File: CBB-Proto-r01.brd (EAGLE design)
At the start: 86.4 x 54.6 mm, 21 parts, among them IC1 IC16_SOIC, IC2 IC6_SOT23, IC4 IC6_SOT23, J1 HEADER_1X23, J10 HEADER_1X3, J11 HEADER_1X3, J12 HEADER_1X3, J13 HEADER_1X8, J14 HEADER_1X8, J15 HEADER_1X8, J16 HEADER_1X8, J2 HEADER_1X23, J3 HEADER_1X23, J4 HEADER_1X23, J5 HEADER_1X4, J6 HEADER_1X4, J7 HEADER_1X4, J8 HEADER_1X4, J9 HEADER_1X3

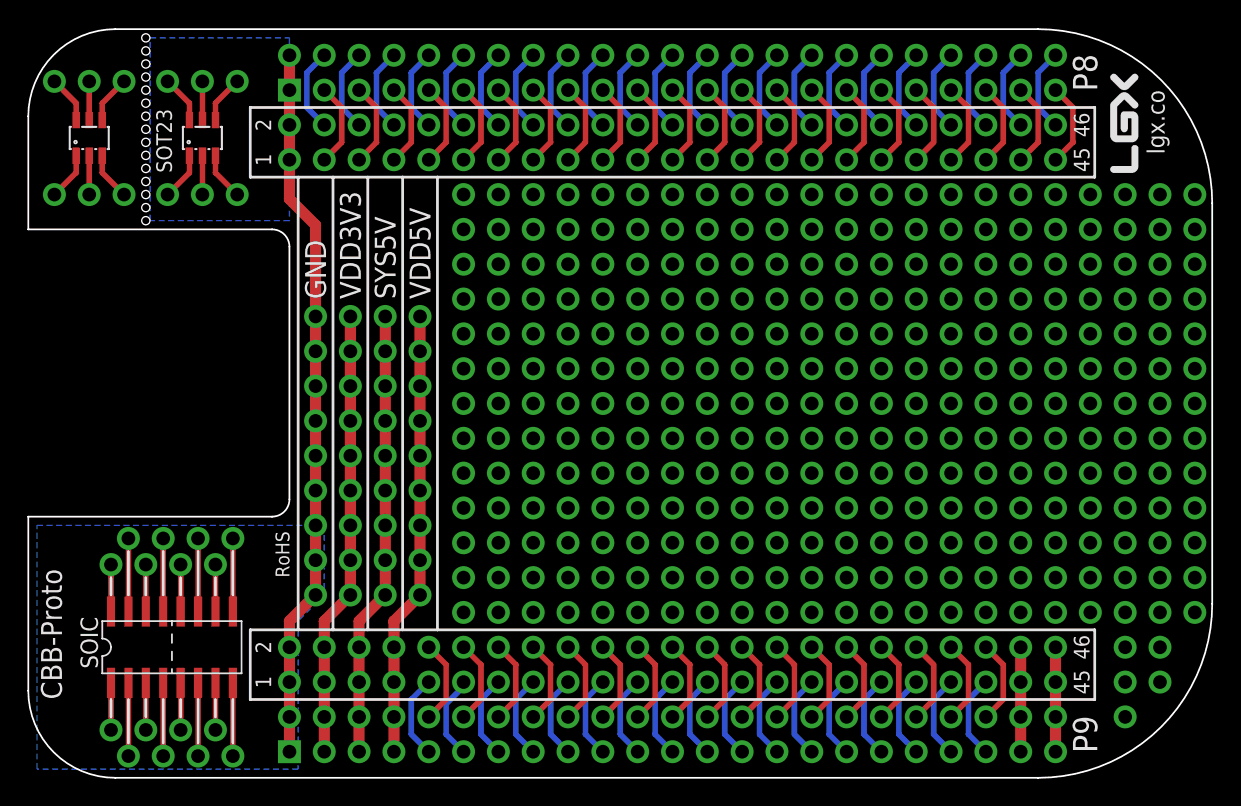
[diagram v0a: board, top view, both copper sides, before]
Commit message: revert to r01
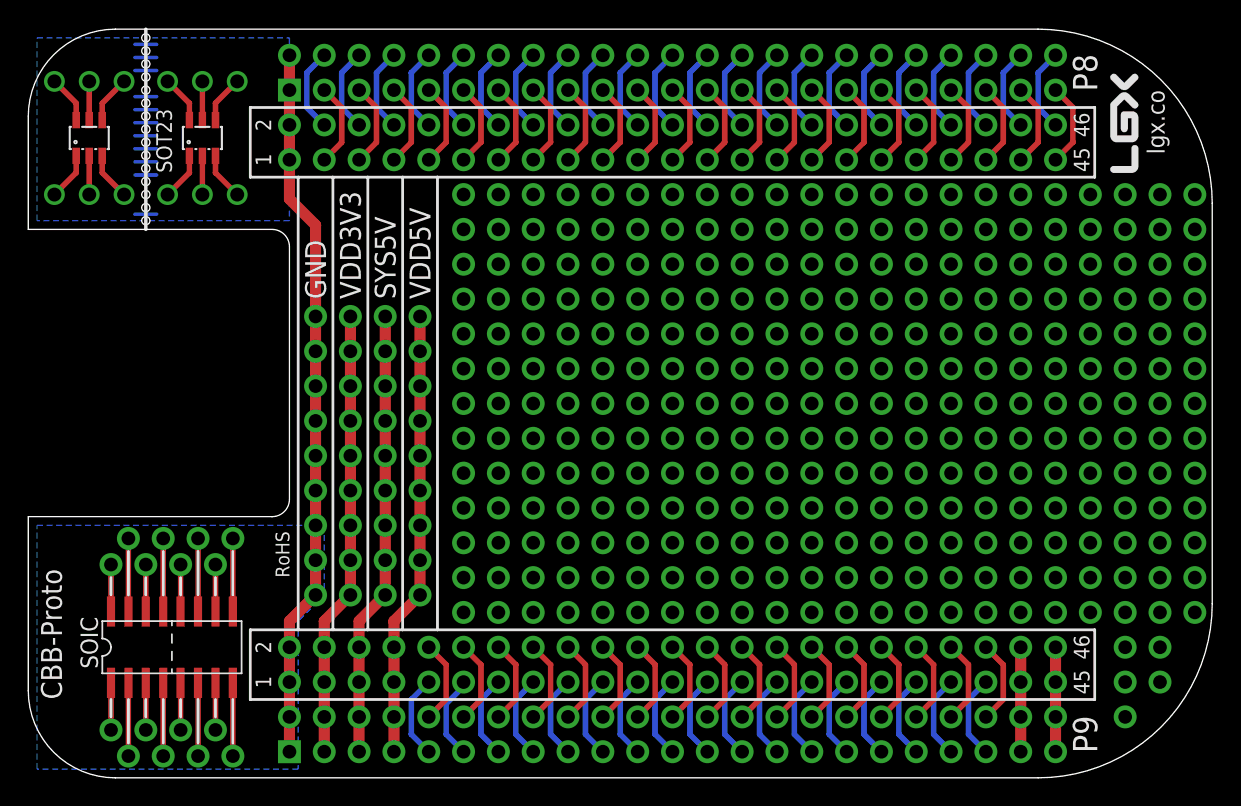
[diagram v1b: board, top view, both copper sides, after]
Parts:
- BB1: value BEAGLEBONECAPE-FULL -> BBH1; device pybbio:BEAGLEBONE_CAPE_FULL -> logic-supply:BB_CAPE
- IC1: device pybbio:SOIC16 -> logic-supply:SOIC16
- IC2, IC4: device pybbio:SOT23-6 -> logic-supply:SOT23-6
- J1, J2, J3, J4: device pybbio:HEADER_1X23 -> logic-supply:HEADER_1X23
- J10, J11, J12, J9: value HEADER_1X3 -> HEADER_1X3_NOSILK; device pybbio:HEADER_1X3 -> logic-supply:HEADER_1X3_NOSILK
- J13, J14, J15, J16: device pybbio:HEADER_1X8 -> logic-supply:HEADER_1X8
- J5, J6, J7, J8: device pybbio:HEADER_1X4 -> logic-supply:HEADER_1X4
- moved J10 2.54 mm to (1.91, 50.8)
- moved J9 2.54 mm to (1.91, 42.5)
- moved J11 2.54 mm to (10.2, 42.5)
- moved J12 2.54 mm to (10.2, 50.8)
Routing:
- net GND: track 67.6 -> 85.1 mm
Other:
- board text added: "1005-0400_r01"
- board text removed: "1005-0400_r02"
- board text removed: "Break off to provide"
- board text removed: "V-score -"
- board text removed: "button/LED access"
